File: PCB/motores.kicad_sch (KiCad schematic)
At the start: 26 parts, among them IC2 IR2175STRPBF, J10 Conn_01x03, J11 Conn_01x03, J12 motor_dc, J9 motor_lineal, K1 G6E, K2 G6E, K3 G6E, K4 G6E, Q1 AO3401A, Q2 AO3401A, Q3 AO3401A, Q4 AO3401A

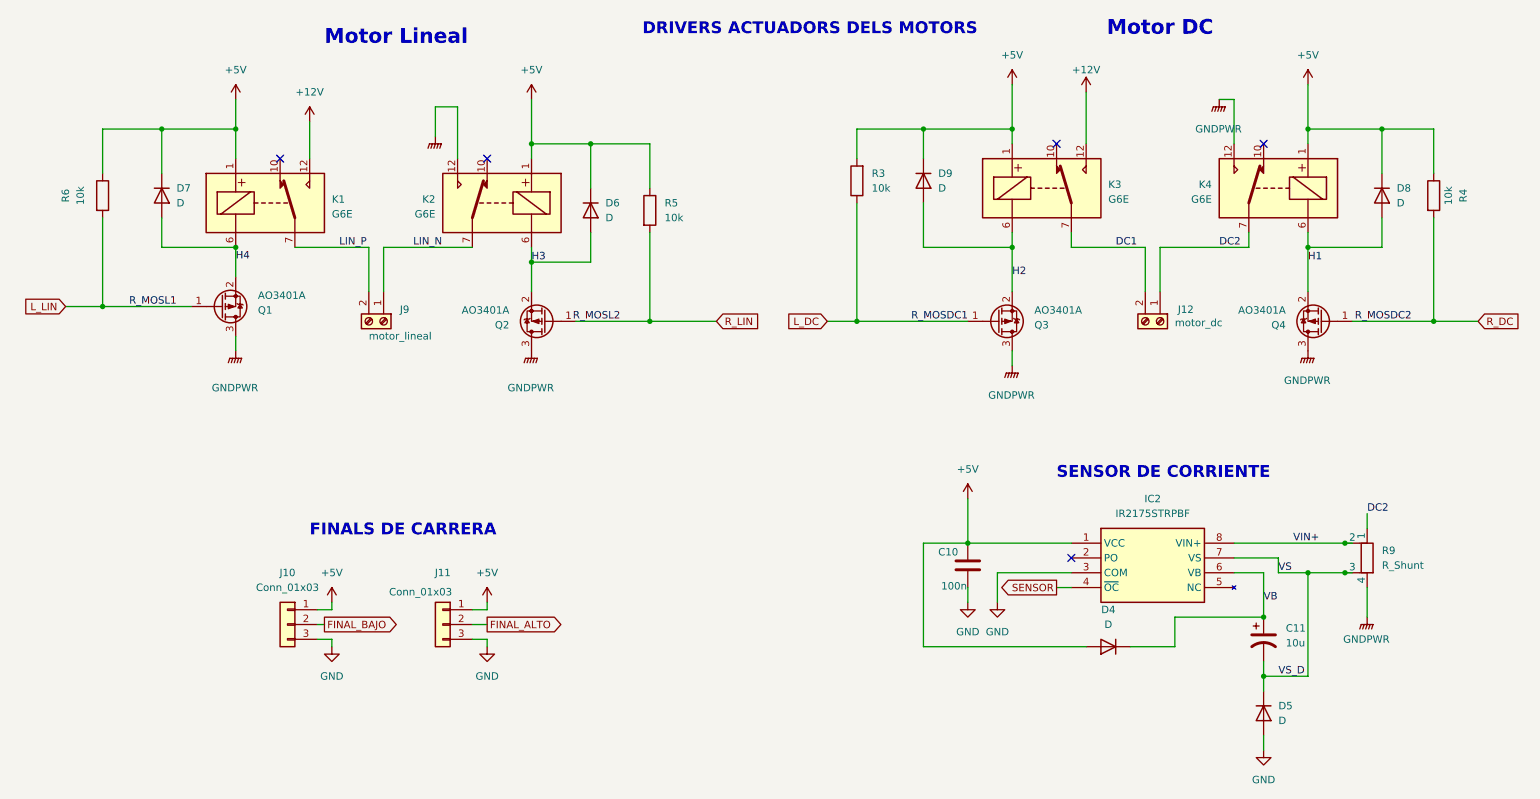
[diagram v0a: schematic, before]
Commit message: Add files via upload
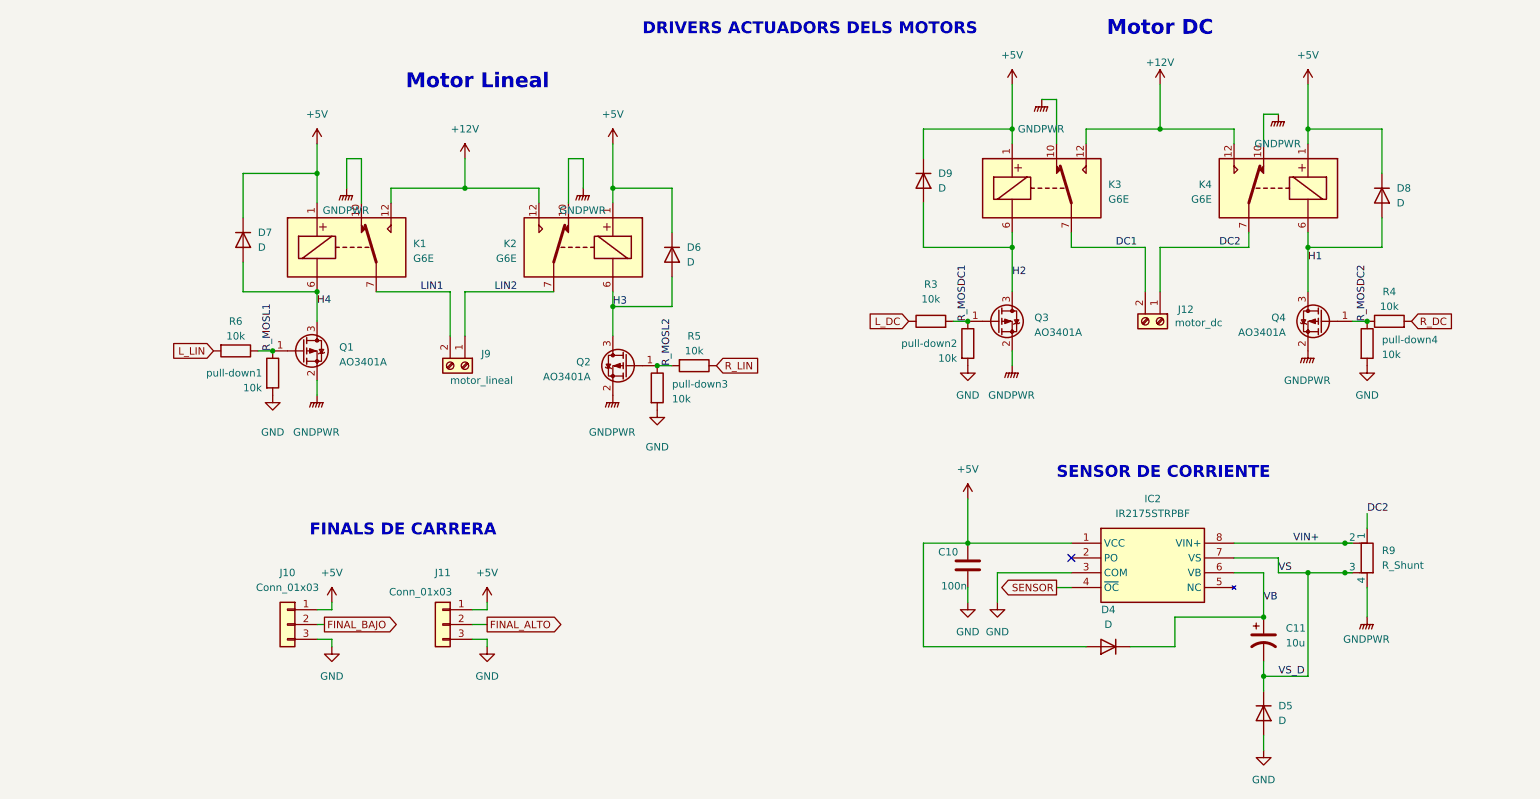
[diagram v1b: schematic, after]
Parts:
- added pull-down1, pull-down2, pull-down3, pull-down4: 10k, Capacitor_SMD:C_1206_3216Metric, symbol Device:R
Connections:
- net +12V: now also K2.12, K4.12
- net +5V: no longer R3.2, R4.1, R5.1, R6.1
- net GND: now also pull-down1.2, pull-down2.2, pull-down3.2, pull-down4.2
- net GNDPWR: now also K1.10, K2.10, K3.10, K4.10, Q1.2 (S), Q2.2 (S), Q3.2 (S), Q4.2 (S); no longer K2.12, K4.12, Q1.3 (D), Q2.3 (D), Q3.3 (D), Q4.3 (D)
- net H1: now also Q4.3 (D); no longer Q4.2 (S)
- net H2: now also Q3.3 (D); no longer Q3.2 (S)
- net H3: now also Q2.3 (D); no longer Q2.2 (S)
- net H4: now also Q1.3 (D); no longer Q1.2 (S)
- net L_DC: no longer Q3.1 (G)
- net L_LIN: no longer Q1.1 (G)
- net R_DC: no longer Q4.1 (G)
- net R_LIN: now also R5.1; no longer Q2.1 (G), R5.2
- net LIN_N renamed LIN2
- net LIN_P renamed LIN1
- new net R_MOSDC1: Q3.1 (G), R3.2, pull-down2.1
- new net R_MOSDC2: Q4.1 (G), R4.1, pull-down4.1
- new net R_MOSL1: Q1.1 (G), R6.1, pull-down1.1
- new net R_MOSL2: Q2.1 (G), R5.2, pull-down3.1
- no-connect marks 5 -> 1
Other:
- moved on the sheet: D6, D7, J9, K1, K2, Q1, Q2, Q4, R3, R4, R5, R6
